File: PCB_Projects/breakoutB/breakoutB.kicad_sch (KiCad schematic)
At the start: 5 parts, among them J1 Conn_01x12_MountingPin, J2 Conn_01x12_MountingPin, J3 Conn_01x05_MountingPin, U1 LDL1117S50R_, U2 LM66100DCKR

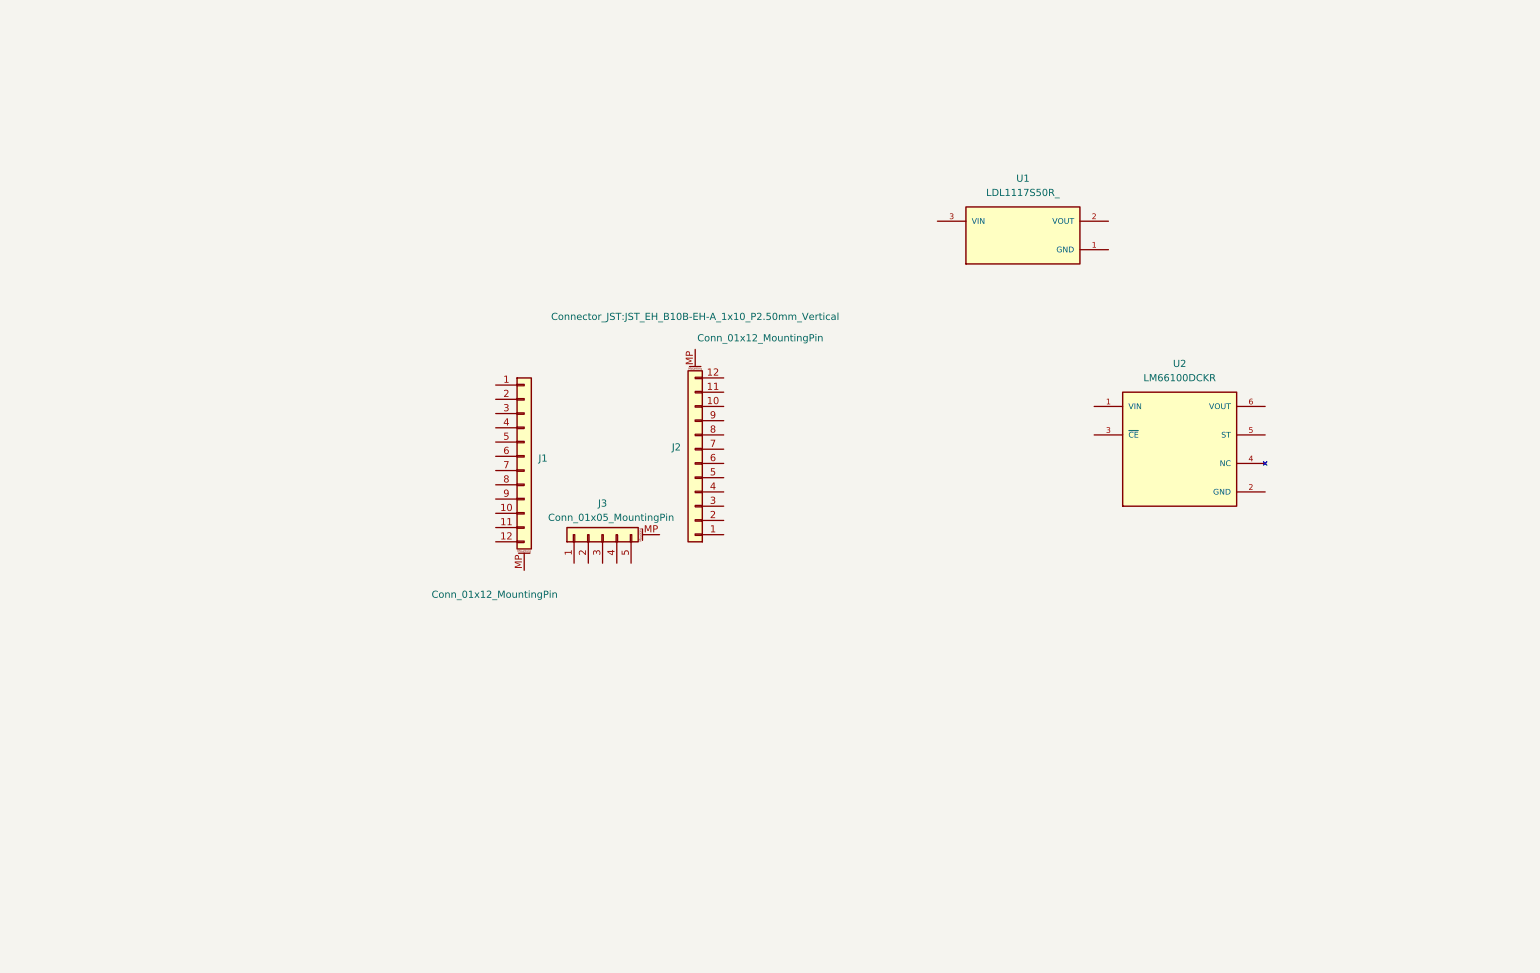
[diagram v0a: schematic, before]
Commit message: feat: PCB & tweak code
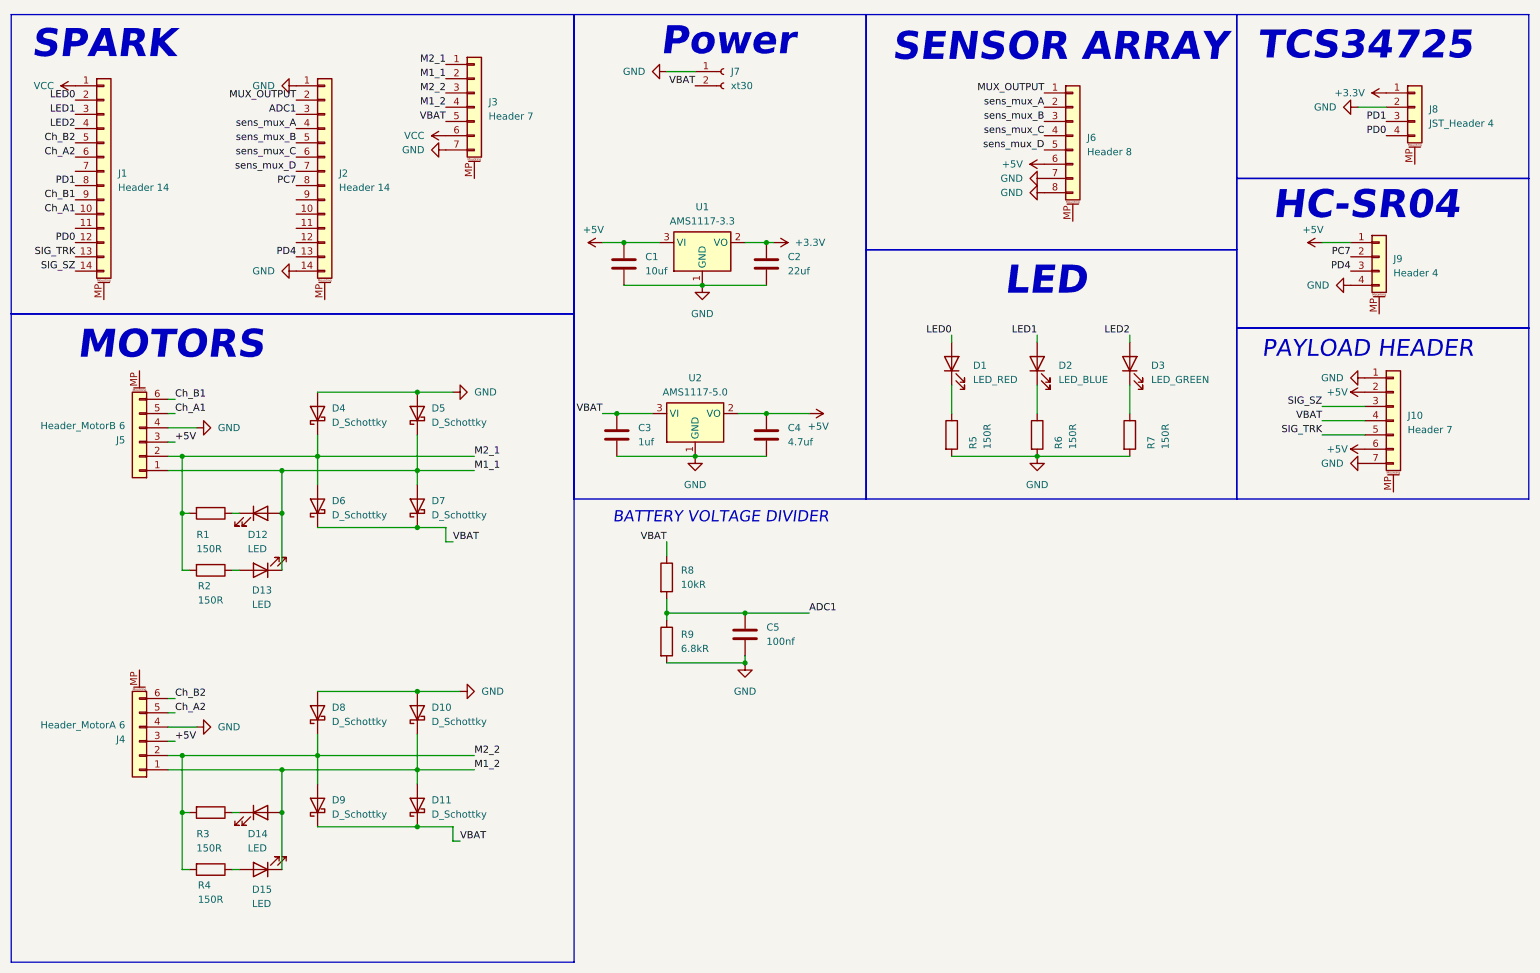
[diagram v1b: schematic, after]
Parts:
- removed J1: Conn_01x12_MountingPin, symbol Connector_Generic_MountingPin:Conn_01x12_MountingPin
- removed J2: Conn_01x12_MountingPin, Connector_JST:JST_EH_B10B-EH-A_1x10_P2.50mm_Vertical, symbol Connector_Generic_MountingPin:Conn_01x12_MountingPin
- removed J3: Conn_01x05_MountingPin, symbol Connector_Generic_MountingPin:Conn_01x05_MountingPin
- removed U1: LDL1117S50R_, LDL1117S50R_:SOT230P700X180-4N, symbol LDL1117S50R_:LDL1117S50R_
- removed U2: LM66100DCKR, LM66100DCKR:SOT65P210X110-6N, symbol LM66100DCKR:LM66100DCKR
- added C1: 10uf, Capacitor_SMD:C_1206_3216Metric, symbol Device:C
- added C2: 22uf, Capacitor_SMD:C_1206_3216Metric, symbol Device:C
- added C3: 1uf, Capacitor_SMD:C_1206_3216Metric, symbol Device:C
- added C4: 4.7uf, Capacitor_SMD:C_1206_3216Metric, symbol Device:C
- added C5: 100nf, Capacitor_SMD:C_1206_3216Metric, symbol Device:C
- added D1: LED_RED, LED_THT:LED_D5.0mm, symbol Device:LED
- added D10, D11, D4, D5, D6, D7, D8, D9: D_Schottky, Diode_SMD:D_SMB, symbol Device:D_Schottky
- added D12, D13, D14, D15: LED, LED_SMD:LED_0603_1608Metric, symbol Device:LED
- added D2: LED_BLUE, LED_THT:LED_D5.0mm, symbol Device:LED
- added D3: LED_GREEN, LED_THT:LED_D5.0mm, symbol Device:LED
- added J1, J2: Header 14, Connector_PinSocket_2.54mm:PinSocket_1x14_P2.54mm_Vertical, symbol Connector_Generic_MountingPin:Conn_01x14_MountingPin
- added J10: Header 7, Connector_JST:JST_EH_B7B-EH-A_1x07_P2.50mm_Vertical, symbol Connector_Generic_MountingPin:Conn_01x07_MountingPin
- added J3: Header 7, Connector_PinSocket_2.54mm:PinSocket_1x07_P2.54mm_Vertical, symbol Connector_Generic_MountingPin:Conn_01x07_MountingPin
- added J4: Header_MotorA 6, Connector_JST:JST_EH_S6B-EH_1x06_P2.50mm_Horizontal, symbol Connector_Generic_MountingPin:Conn_01x06_MountingPin
- added J5: Header_MotorB 6, Connector_JST:JST_EH_S6B-EH_1x06_P2.50mm_Horizontal, symbol Connector_Generic_MountingPin:Conn_01x06_MountingPin
- added J6: Header 8, Connector_PinSocket_2.54mm:PinSocket_1x08_P2.54mm_Vertical, symbol Connector_Generic_MountingPin:Conn_01x08_MountingPin
- added J7: xt30, Connector_AMASS:AMASS_XT30PW-M_1x02_P2.50mm_Horizontal, symbol Connector:Conn_01x02_Socket
- added J8: JST_Header 4, Connector_JST:JST_PH_S4B-PH-K_1x04_P2.00mm_Horizontal, symbol Connector_Generic_MountingPin:Conn_01x04_MountingPin
- added J9: Header 4, Connector_PinSocket_2.54mm:PinSocket_1x04_P2.54mm_Vertical, symbol Connector_Generic_MountingPin:Conn_01x04_MountingPin
- added R1, R2, R3, R4, R5, R6, R7: 150R, Resistor_SMD:R_0603_1608Metric, symbol Device:R
- added R8: 10kR, Resistor_SMD:R_0603_1608Metric, symbol Device:R
- added R9: 6.8kR, Resistor_SMD:R_0603_1608Metric, symbol Device:R
- added U1: AMS1117-3.3, Package_TO_SOT_SMD:SOT-223-3_TabPin2, symbol Regulator_Linear:AMS1117-3.3
- added U2: AMS1117-5.0, Package_TO_SOT_SMD:SOT-223-3_TabPin2, symbol Regulator_Linear:AMS1117-5.0
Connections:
- new net: D12.1 (K), R1.1
- new net: D14.1 (K), R3.1
- new net: D3.1 (K), R7.1
- new net: D15.2 (A), R4.1
- new net: D13.2 (A), R2.1
- new net: D1.1 (K), R5.1
- new net: D2.1 (K), R6.1
- new net +3.3V: C2.1, J8.1 (Pin_1), U1.2 (VO)
- new net +5V: C1.1, C4.1, J10.2 (Pin_2), J10.6 (Pin_6), J4.3 (Pin_3), J5.3 (Pin_3), J6.6 (Pin_6), J9.1 (Pin_1), U1.3 (VI), U2.2 (VO)
- new net ADC1: C5.1, J2.3 (Pin_3), R8.2, R9.1
- new net Ch_A1: J1.10 (Pin_10), J5.5 (Pin_5)
- new net Ch_A2: J1.6 (Pin_6), J4.5 (Pin_5)
- new net Ch_B1: J1.9 (Pin_9), J5.6 (Pin_6)
- new net Ch_B2: J1.5 (Pin_5), J4.6 (Pin_6)
- new net GND: C1.2, C2.2, C3.2, C4.2, C5.2, D10.2 (A), D4.2 (A), D5.2 (A), D8.2 (A), J10.1 (Pin_1), J10.7 (Pin_7), J2.1 (Pin_1), J2.14 (Pin_14), J3.7 (Pin_7), J4.4 (Pin_4), J5.4 (Pin_4), J6.7 (Pin_7), J6.8 (Pin_8), J7.1 (Pin_1), J8.2 (Pin_2), J9.4 (Pin_4), R5.2, R6.2, R7.2, R9.2, U1.1 (GND), U2.1 (GND)
- new net LED0: D1.2 (A), J1.2 (Pin_2)
- new net LED1: D2.2 (A), J1.3 (Pin_3)
- new net LED2: D3.2 (A), J1.4 (Pin_4)
- new net M1_1: D12.2 (A), D13.1 (K), D5.1 (K), D7.2 (A), J3.2 (Pin_2), J5.1 (Pin_1)
- new net M1_2: D10.1 (K), D11.2 (A), D14.2 (A), D15.1 (K), J3.4 (Pin_4), J4.1 (Pin_1)
- new net M2_1: D4.1 (K), D6.2 (A), J3.1 (Pin_1), J5.2 (Pin_2), R1.2, R2.2
- new net M2_2: D8.1 (K), D9.2 (A), J3.3 (Pin_3), J4.2 (Pin_2), R3.2, R4.2
- new net MUX_OUTPUT: J2.2 (Pin_2), J6.1 (Pin_1)
- new net PC7: J2.8 (Pin_8), J9.2 (Pin_2)
- new net PD0: J1.12 (Pin_12), J8.4 (Pin_4)
- new net PD1: J1.8 (Pin_8), J8.3 (Pin_3)
- new net PD4: J2.13 (Pin_13), J9.3 (Pin_3)
- new net SIG_SZ: J1.14 (Pin_14), J10.3 (Pin_3)
- new net SIG_TRK: J1.13 (Pin_13), J10.5 (Pin_5)
- new net VBAT: C3.1, D11.1 (K), D6.1 (K), D7.1 (K), D9.1 (K), J10.4 (Pin_4), J3.5 (Pin_5), J7.2 (Pin_2), R8.1, U2.3 (VI)
- new net VCC: J1.1 (Pin_1), J3.6 (Pin_6)
- new net sens_mux_A: J2.4 (Pin_4), J6.2 (Pin_2)
- new net sens_mux_B: J2.5 (Pin_5), J6.3 (Pin_3)
- new net sens_mux_C: J2.6 (Pin_6), J6.4 (Pin_4)
- new net sens_mux_D: J2.7 (Pin_7), J6.5 (Pin_5)
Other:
- note added: "BATTERY VOLTAGE DIVIDER"
- note added: "HC-SR04"
- note added: "LED"
- note added: "MOTORS"
- note added: "PAYLOAD HEADER"
- note added: "Power"
- note added: "SENSOR ARRAY"
- note added: "SPARK"
- note added: "TCS34725"
